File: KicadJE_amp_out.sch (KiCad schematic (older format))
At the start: 36 parts

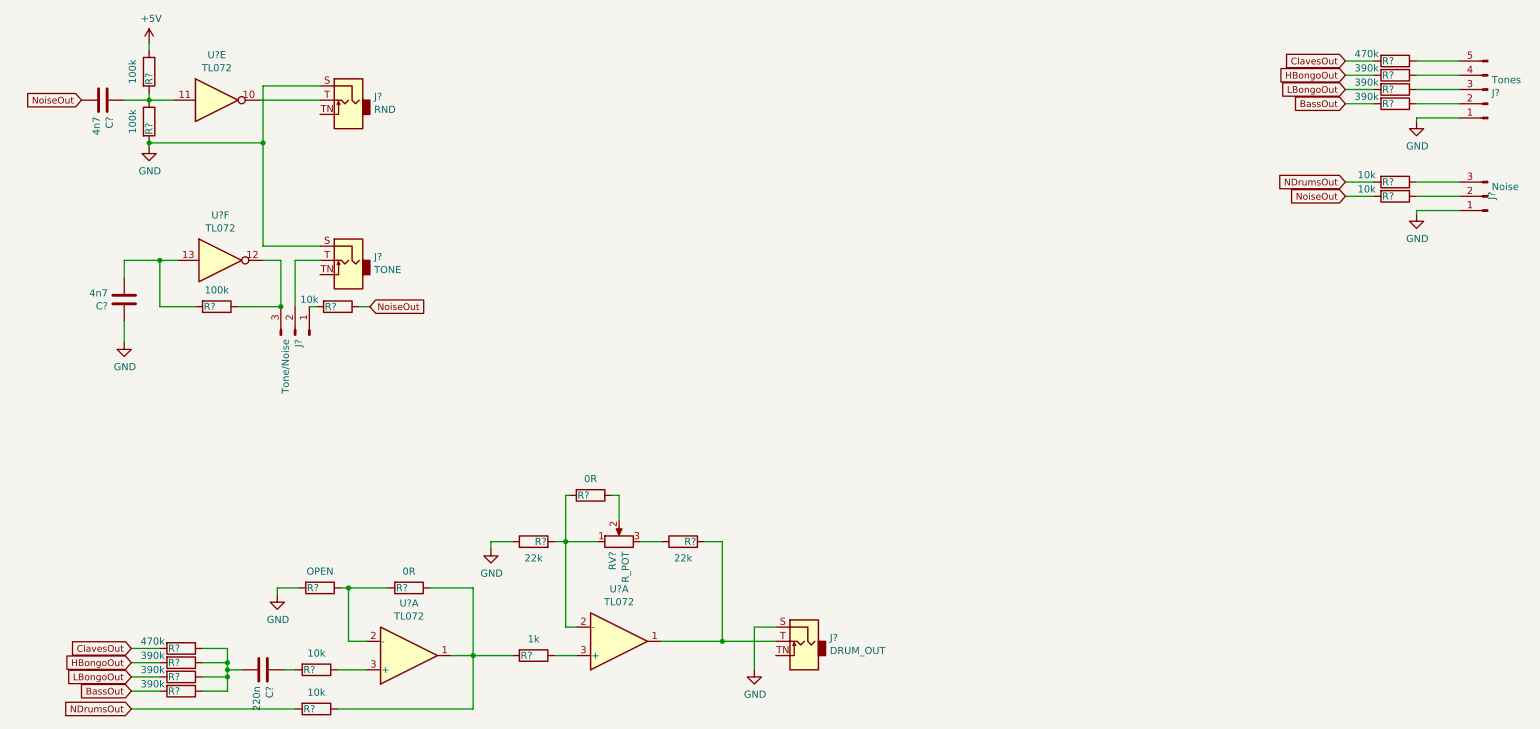
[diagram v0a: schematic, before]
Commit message: Annotate
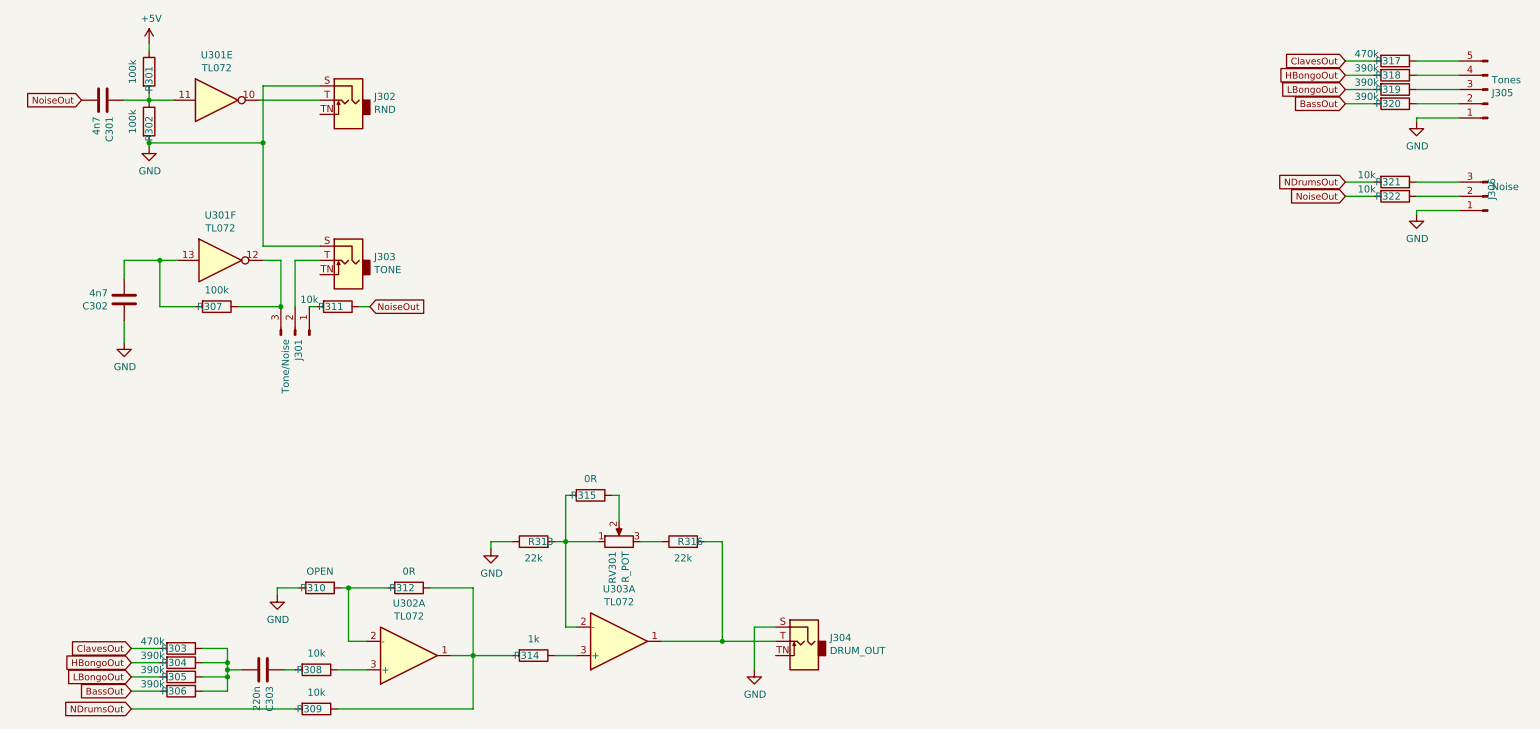
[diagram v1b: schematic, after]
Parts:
- gave numbers to parts that had none: 35
